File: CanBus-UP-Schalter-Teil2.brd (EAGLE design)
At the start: 42.2 x 37.2 mm, 28 parts, among them IC1 LM2937IMP-5.0, IC2 MEGA8-AI, IC3 MCP2515T-I/SO, Q1 EUROQUARTZ-MMJ, Q2 EUROQUARTZ-MMJ, Q3 BC847ASMD, Q4 BC847ASMD, U1 MCP2562-E/SN

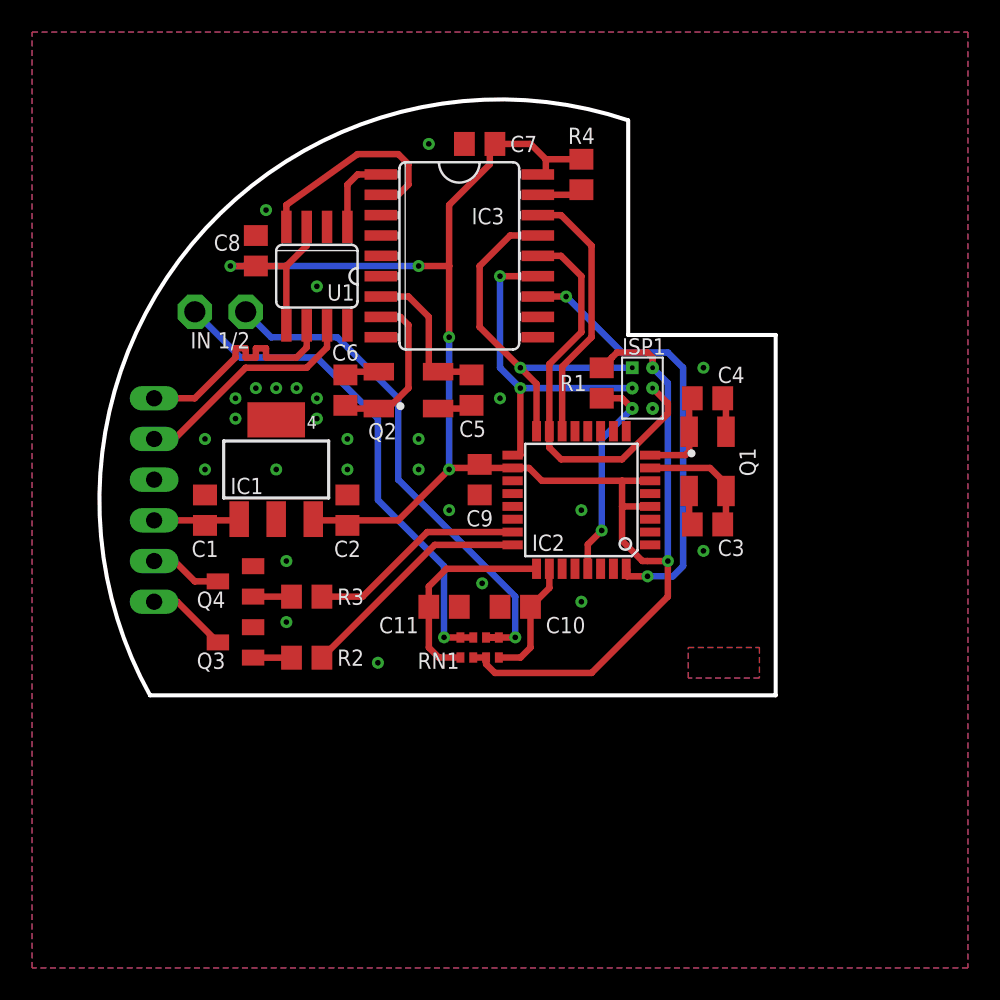
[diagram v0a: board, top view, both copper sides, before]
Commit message: CanBus-UP-Schalter fertiggestellt
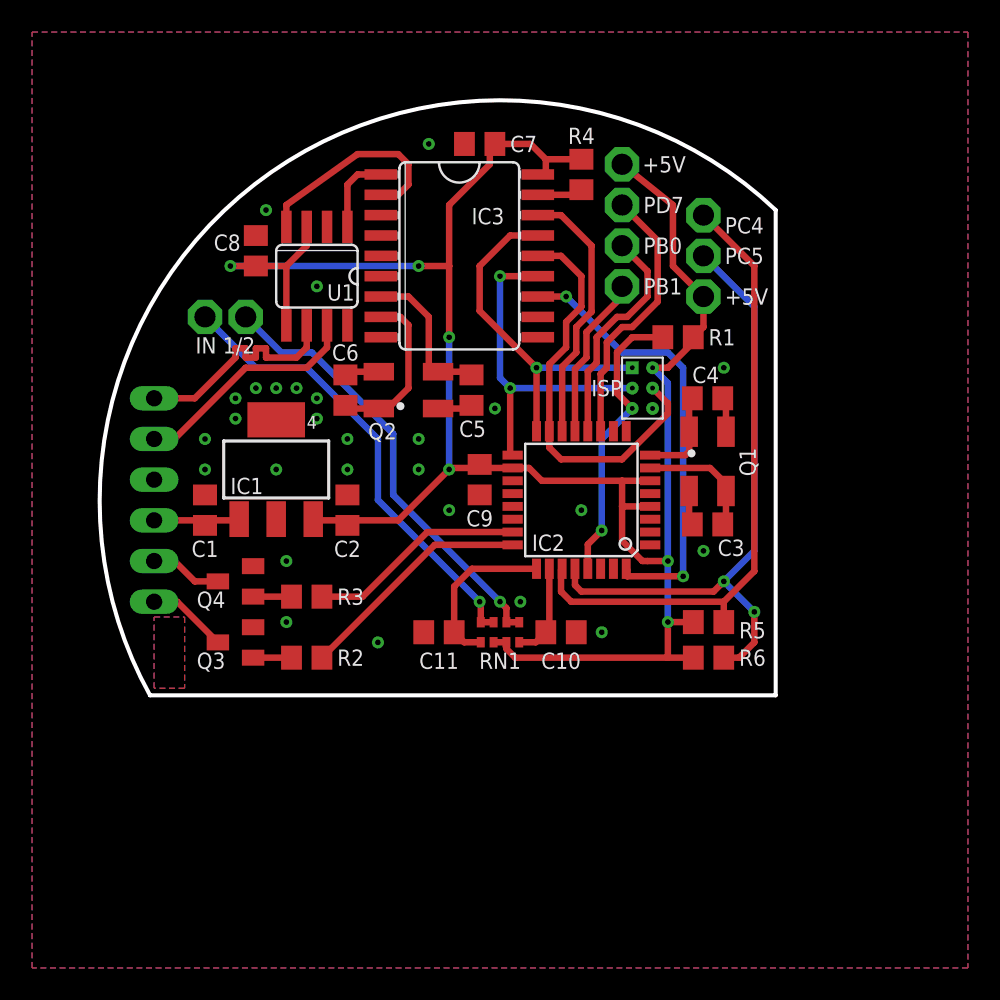
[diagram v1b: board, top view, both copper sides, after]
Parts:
- added +5V, +5V1, PB0, PB1, PC4, PC5, PD7: LSP13, solpad:LSP13
- added R5, R6: 4k7, rcl:R0805
- moved R1 5.55 mm to (11.1, 10.2), turned to 0 degrees
- moved C10 3.27 mm to (3.81, -8.26), turned to 0 degrees
- moved C11 1.62 mm to (-3.81, -8.26), turned to 180 degrees
- moved RN1 1.59 mm to (0.00, -8.26)
- moved LSP1 0.71 mm to (-18.4, 11.4)
- moved LSP2 0.32 mm to (-15.9, 11.4)
- renumbered ISP1 to ISP
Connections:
- new net N$10: IC2.28, PC5.MP, R6.1
- new net N$11: IC2.27, PC4.MP, R5.1
- new net N$7: IC2.13, PB1.MP
- new net N$8: IC2.12, PB0.MP
- new net N$9: IC2.11, PD7.MP
- net +5V: now also +5V.MP, +5V1.MP, R5.2, R6.2
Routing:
- net N$10: track 0.00 -> 40.1 mm, vias 0 -> 2
- net N$11: track 0.00 -> 39.4 mm
- net N$9: track 0.00 -> 16.9 mm
- net +5V: track 118.8 -> 135.2 mm, vias 5 -> 6
- net N$8: track 0.00 -> 14.2 mm
- net N$7: track 0.00 -> 10.3 mm
- net RST: track 13.3 -> 18.3 mm
- net N$6: track 32.3 -> 27.7 mm
- net IN1: track 13.2 -> 10.4 mm
- net N$5: track 31.4 -> 28.9 mm
- net IN2: track 7.64 -> 5.97 mm
- net MISO: track 23.2 -> 22.2 mm
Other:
- board size 42.2 x 37.2 mm -> 42.2 x 37.1 mm
- board text added: "+5V"
